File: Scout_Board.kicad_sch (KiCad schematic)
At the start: 3 parts, among them U1 ESP32-S3-DEVKITC-1U-N8R2

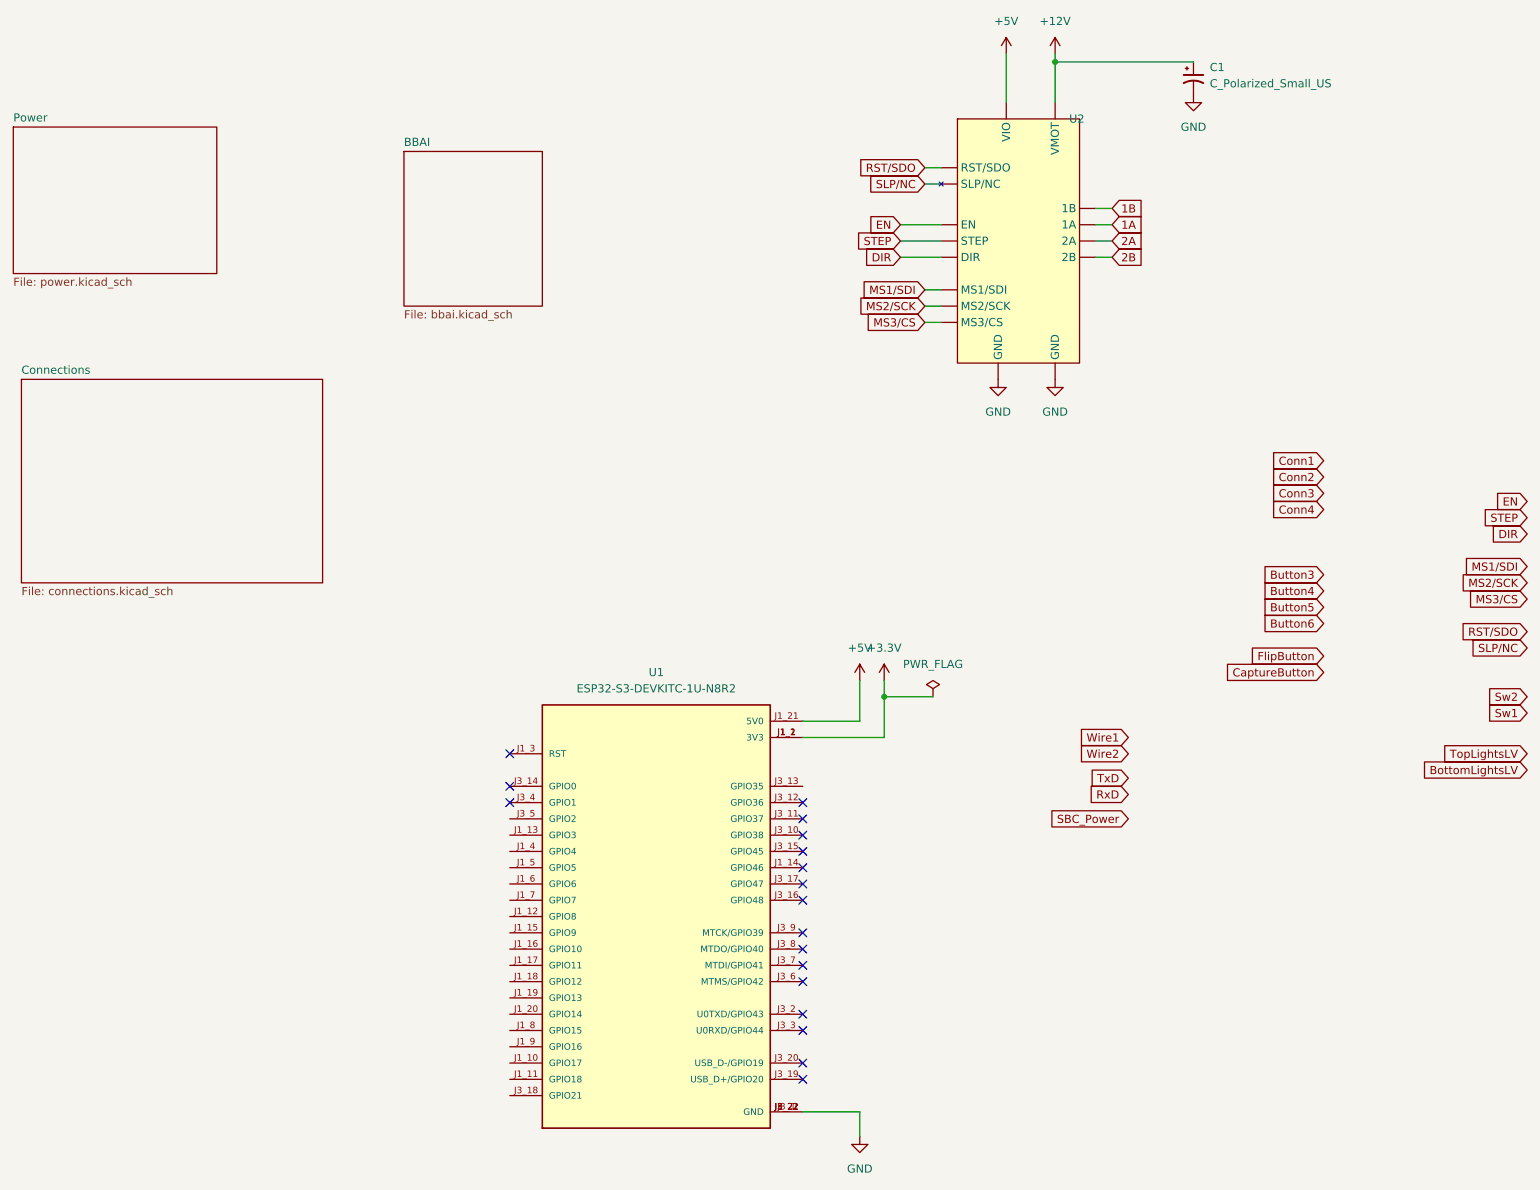
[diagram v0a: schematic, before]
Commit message: New board test
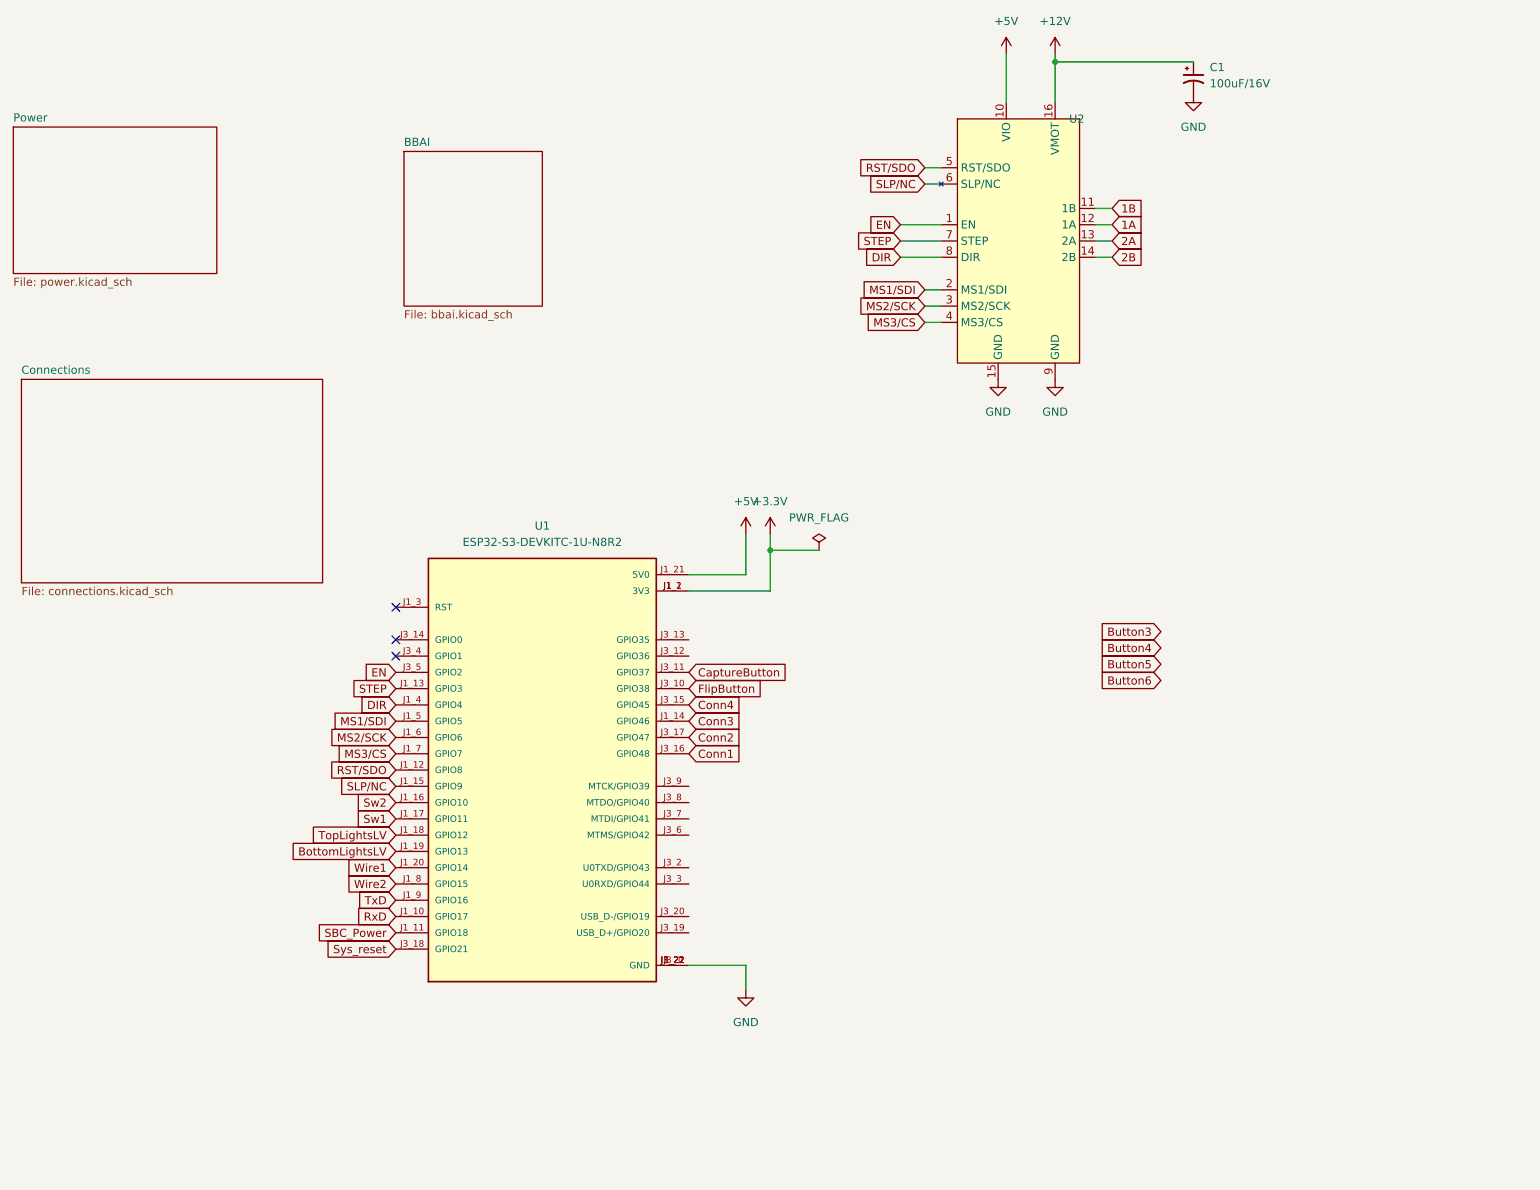
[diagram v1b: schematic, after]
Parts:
- C1: value C_Polarized_Small_US -> 100uF/16V; footprint (none) -> Capacitor_SMD:CP_Elec_6.3x5.9
- U1: footprint Downloaded_footprints:XCVR_ESP32-S3-DEVKITC-1U-N8R2 -> ESP32-S3-DEVKITC-1-N8R2:XCVR_ESP32-S3-DEVKITC-1-N8R2
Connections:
- net +12V: now also U2.16 (VMOT); no longer U2. (SLP/NC)
- net +5V: now also U2.10 (VIO); no longer U2. (SLP/NC)
- net 1A: now also U2.12 (1A); no longer U2. (SLP/NC)
- net 1B: now also U2.11 (1B); no longer U2. (SLP/NC)
- net 2A: now also U2.13 (2A); no longer U2. (SLP/NC)
- net 2B: now also U2.14 (2B); no longer U2. (SLP/NC)
- net BottomLightsLV: now also U1.J1_19 (GPIO13)
- net CaptureButton: now also U1.J3_11 (GPIO37)
- net Conn1: now also U1.J3_16 (GPIO48)
- net Conn2: now also U1.J3_17 (GPIO47)
- net Conn3: now also U1.J1_14 (GPIO46)
- net Conn4: now also U1.J3_15 (GPIO45)
- net DIR: now also U1.J1_4 (GPIO4), U2.8 (DIR); no longer U2. (SLP/NC)
- net EN: now also U1.J3_5 (GPIO2), U2.1 (EN); no longer U2. (SLP/NC)
- net FlipButton: now also U1.J3_10 (GPIO38)
- net GND: now also U2.15 (GND), U2.9 (GND); no longer U2. (SLP/NC)
- net MS1/SDI: now also U1.J1_5 (GPIO5), U2.2 (MS1/SDI); no longer U2. (SLP/NC)
- net MS2/SCK: now also U1.J1_6 (GPIO6), U2.3 (MS2/SCK); no longer U2. (SLP/NC)
- net MS3/CS: now also U1.J1_7 (GPIO7), U2.4 (MS3/CS); no longer U2. (SLP/NC)
- net RST/SDO: now also U1.J1_12 (GPIO8), U2.5 (RST/SDO); no longer U2. (SLP/NC)
- net RxD: now also U1.J1_10 (GPIO17)
- net SBC_Power: now also U1.J1_11 (GPIO18)
- net SLP/NC: now also U1.J1_15 (GPIO9), U2.6 (SLP/NC); no longer U2. (SLP/NC)
- net STEP: now also U1.J1_13 (GPIO3), U2.7 (STEP); no longer U2. (SLP/NC)
- net Sw1: now also U1.J1_17 (GPIO11)
- net Sw2: now also U1.J1_16 (GPIO10)
- net TopLightsLV: now also U1.J1_18 (GPIO12)
- net TxD: now also U1.J1_9 (GPIO16)
- net Wire1: now also U1.J1_20 (GPIO14)
- net Wire2: now also U1.J1_8 (GPIO15)
- net Sys_reset: now reaches U1.J3_18 (GPIO21)
- no-connect marks 18 -> 3
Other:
- moved on the sheet: U1

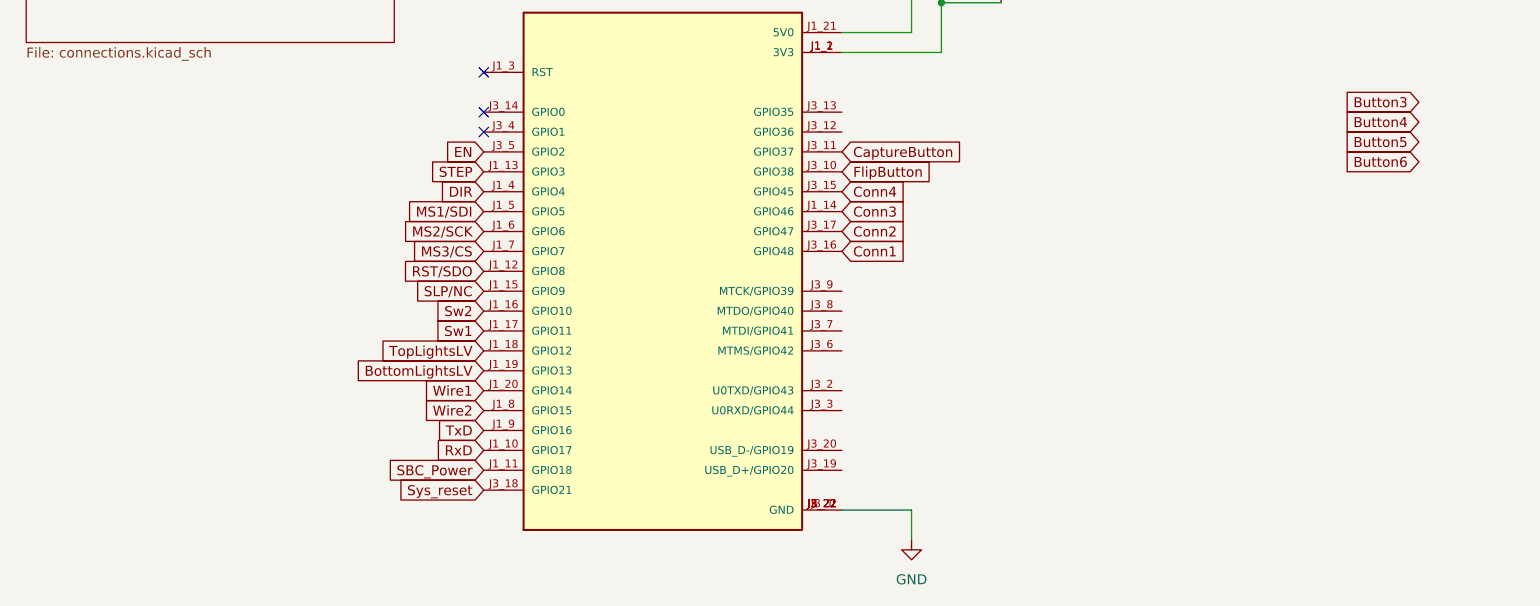
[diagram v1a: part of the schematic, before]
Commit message: Layout changes
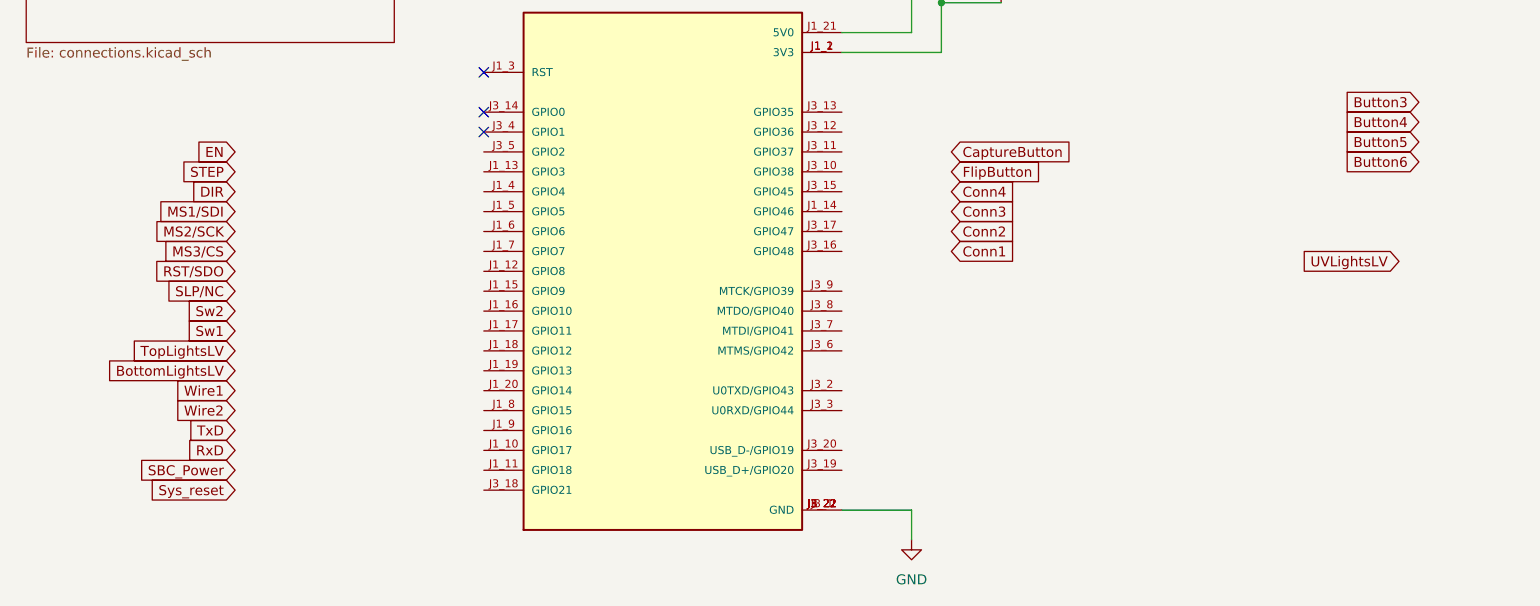
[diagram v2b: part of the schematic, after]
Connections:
- net BottomLightsLV: no longer U1.J1_19 (GPIO13)
- net CaptureButton: no longer U1.J3_11 (GPIO37)
- net Conn1: no longer U1.J3_16 (GPIO48)
- net Conn2: no longer U1.J3_17 (GPIO47)
- net Conn3: no longer U1.J1_14 (GPIO46)
- net Conn4: no longer U1.J3_15 (GPIO45)
- net DIR: no longer U1.J1_4 (GPIO4)
- net EN: no longer U1.J3_5 (GPIO2)
- net FlipButton: no longer U1.J3_10 (GPIO38)
- net MS1/SDI: no longer U1.J1_5 (GPIO5)
- net MS2/SCK: no longer U1.J1_6 (GPIO6)
- net MS3/CS: no longer U1.J1_7 (GPIO7)
- net RST/SDO: no longer U1.J1_12 (GPIO8)
- net RxD: no longer U1.J1_10 (GPIO17)
- net SBC_Power: no longer U1.J1_11 (GPIO18)
- net SLP/NC: no longer U1.J1_15 (GPIO9)
- net STEP: no longer U1.J1_13 (GPIO3)
- net Sw1: no longer U1.J1_17 (GPIO11)
- net Sw2: no longer U1.J1_16 (GPIO10)
- net Sys_reset: no longer U1.J3_18 (GPIO21)
- net TopLightsLV: no longer U1.J1_18 (GPIO12)
- net TxD: no longer U1.J1_9 (GPIO16)
- net Wire1: no longer U1.J1_20 (GPIO14)
- net Wire2: no longer U1.J1_8 (GPIO15)
